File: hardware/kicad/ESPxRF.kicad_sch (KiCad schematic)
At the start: 39 parts, among them J1 USB_C_Receptacle_USB2.0, J2 ANT, U1 USBLC6-2SC6, U2 NCP115ASN330T2G, U3 ESP32-S3, U4 NRF24L01, Y1 Crystal_GND24_Small

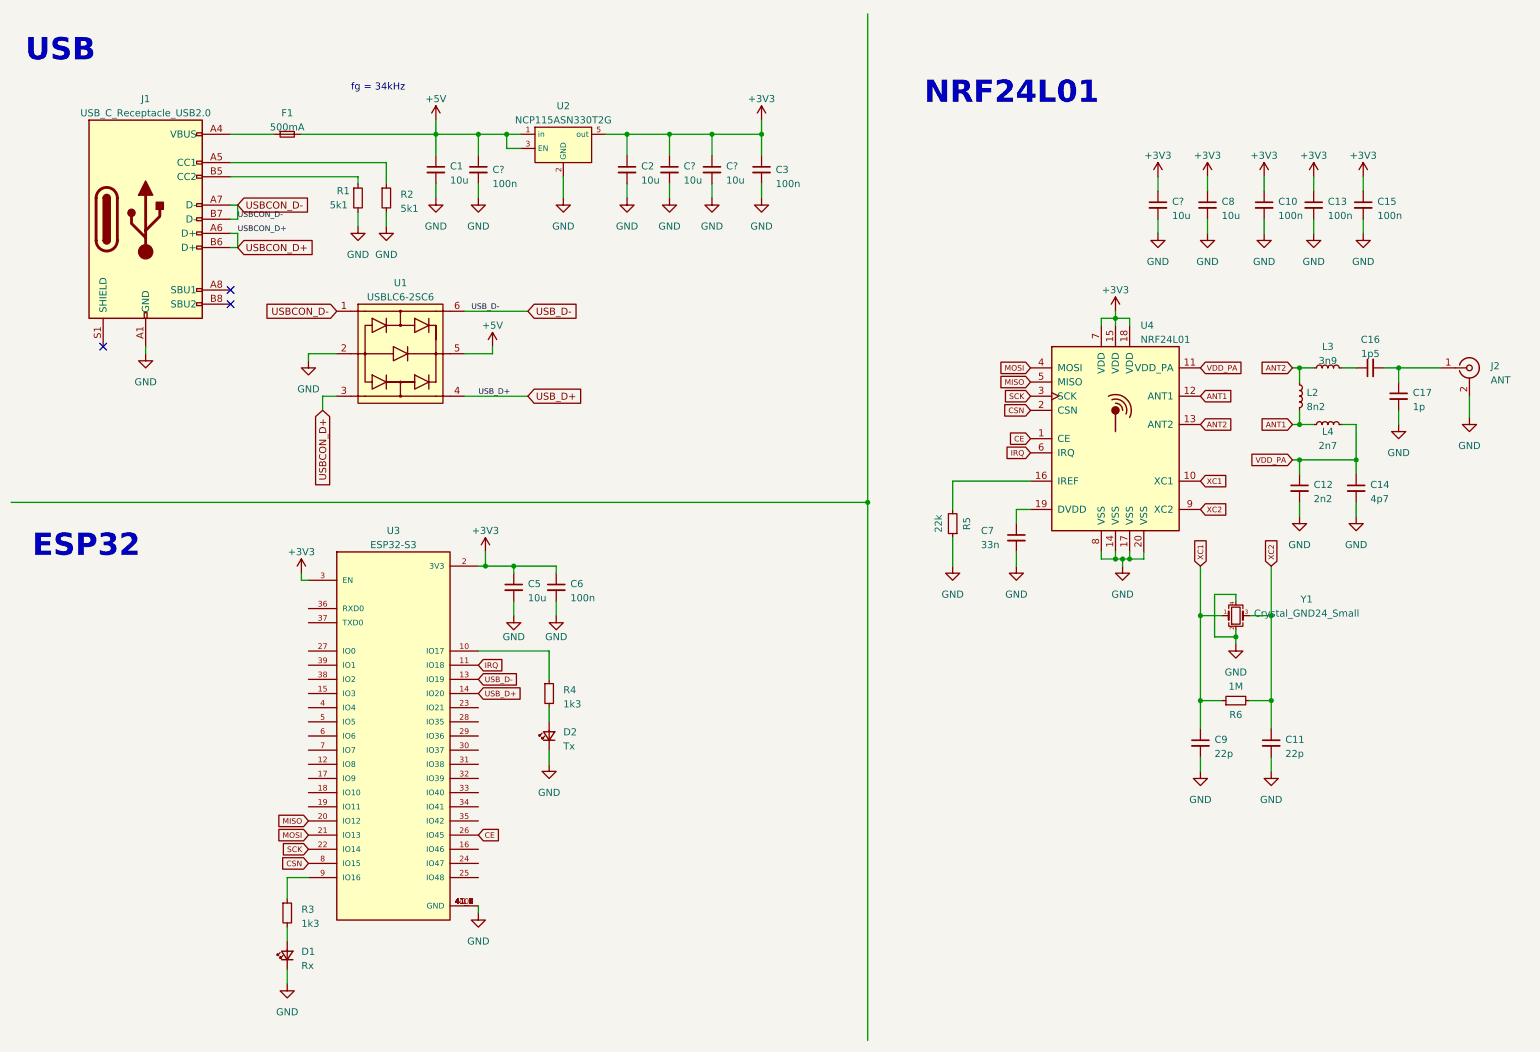
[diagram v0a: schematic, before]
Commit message: V2
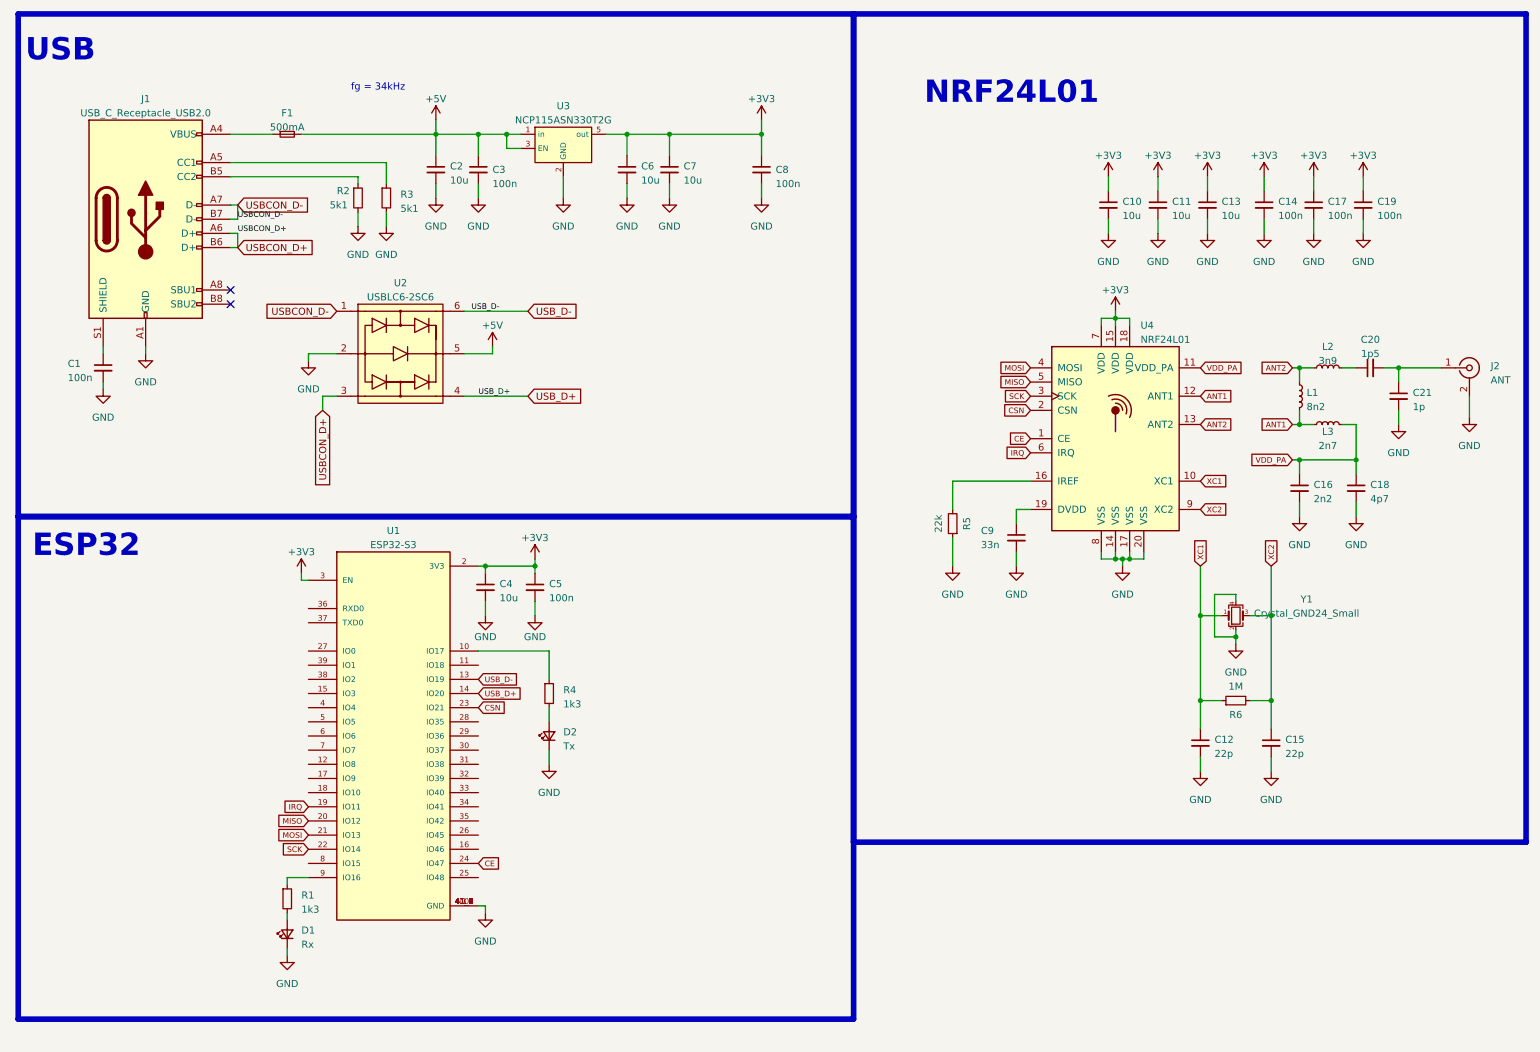
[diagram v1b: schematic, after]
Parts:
- removed C?: 10u, Capacitor_SMD:C_0805_2012Metric_Pad1.18x1.45mm_HandSolder, symbol Device:C_Small
- added C1: 100n, Capacitor_SMD:C_0603_1608Metric_Pad1.08x0.95mm_HandSolder, symbol Device:C_Small
- added C10: 10u, Capacitor_SMD:C_0805_2012Metric_Pad1.18x1.45mm_HandSolder, symbol Device:C_Small
- C12: renamed from C9; footprint Capacitor_SMD:C_0402_1005Metric_Pad0.74x0.62mm_HandSolder -> Capacitor_SMD:C_0603_1608Metric_Pad1.08x0.95mm_HandSolder
- C14: renamed from C10; footprint Capacitor_SMD:C_0402_1005Metric_Pad0.74x0.62mm_HandSolder -> Capacitor_SMD:C_0603_1608Metric_Pad1.08x0.95mm_HandSolder
- C15: renamed from C11; footprint Capacitor_SMD:C_0402_1005Metric_Pad0.74x0.62mm_HandSolder -> Capacitor_SMD:C_0603_1608Metric_Pad1.08x0.95mm_HandSolder
- C17: renamed from C13; footprint Capacitor_SMD:C_0402_1005Metric_Pad0.74x0.62mm_HandSolder -> Capacitor_SMD:C_0603_1608Metric_Pad1.08x0.95mm_HandSolder
- C19: renamed from C15; footprint Capacitor_SMD:C_0402_1005Metric_Pad0.74x0.62mm_HandSolder -> Capacitor_SMD:C_0603_1608Metric_Pad1.08x0.95mm_HandSolder
- C4: renamed from C5; footprint Capacitor_SMD:C_0603_1608Metric_Pad1.08x0.95mm_HandSolder -> Capacitor_SMD:C_0805_2012Metric_Pad1.18x1.45mm_HandSolder
- C9: renamed from C7; footprint Capacitor_SMD:C_0402_1005Metric_Pad0.74x0.62mm_HandSolder -> Capacitor_SMD:C_0603_1608Metric_Pad1.08x0.95mm_HandSolder
- J2: footprint Connector_Coaxial:SMA_Samtec_SMA-J-P-X-ST-EM1_EdgeMount -> Connector_Coaxial:SMA_Samtec_SMA-J-P-H-ST-EM1_EdgeMount
- R5, R6: footprint Resistor_SMD:R_0402_1005Metric_Pad0.72x0.64mm_HandSolder -> Resistor_SMD:R_0603_1608Metric_Pad0.98x0.95mm_HandSolder
- U1: renamed from U3; footprint ESP32:XCVR_ESP32S3WROOM1N8R8 -> ESP32-S3-WROOM:XCVR_ESP32S3WROOM1N8R8
- gave numbers to parts that had none: 3
- renumbered C8 to C13, C12 to C16, C14 to C18, C1 to C2, C16 to C20, C17 to C21, C6 to C5, C2 to C6, C3 to C8, L2 to L1, L3 to L2, L4 to L3, R3 to R1, R1 to R2, R2 to R3, U1 to U2, U2 to U3
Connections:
- net +3V3: now also C10.1
- net CE: now also U1.24 (IO47); no longer U1.26 (IO45)
- net CSN: now also U1.23 (IO21); no longer U1.8 (IO15)
- net GND: now also C1.2, C10.2
- net IRQ: now also U1.19 (IO11); no longer U1.11 (IO18)
- net at J1.S1 (SHIELD): now also C1.1
- no-connect marks 3 -> 2
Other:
- moved on the sheet: C4, C5, D1, R1
